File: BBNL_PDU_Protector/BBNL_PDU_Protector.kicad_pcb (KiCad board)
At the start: 2 copper layers, 107.3 x 39.4 mm, 20 parts, among them J1 1720796, J2 1708381

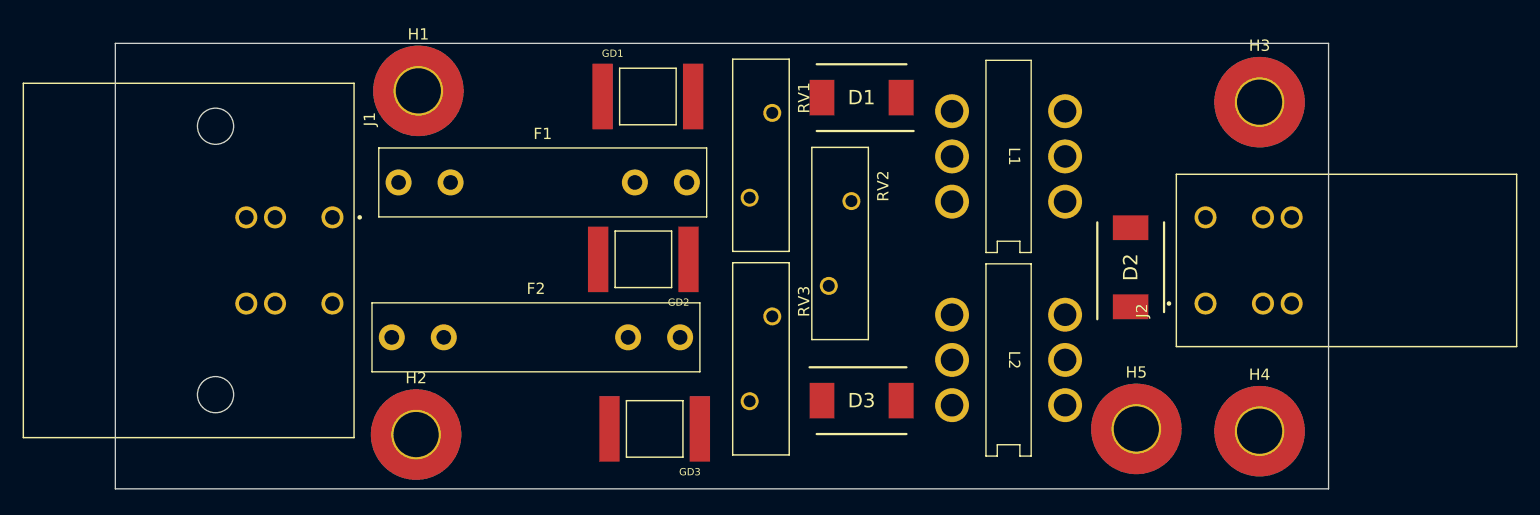
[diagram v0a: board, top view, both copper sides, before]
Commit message: second commit
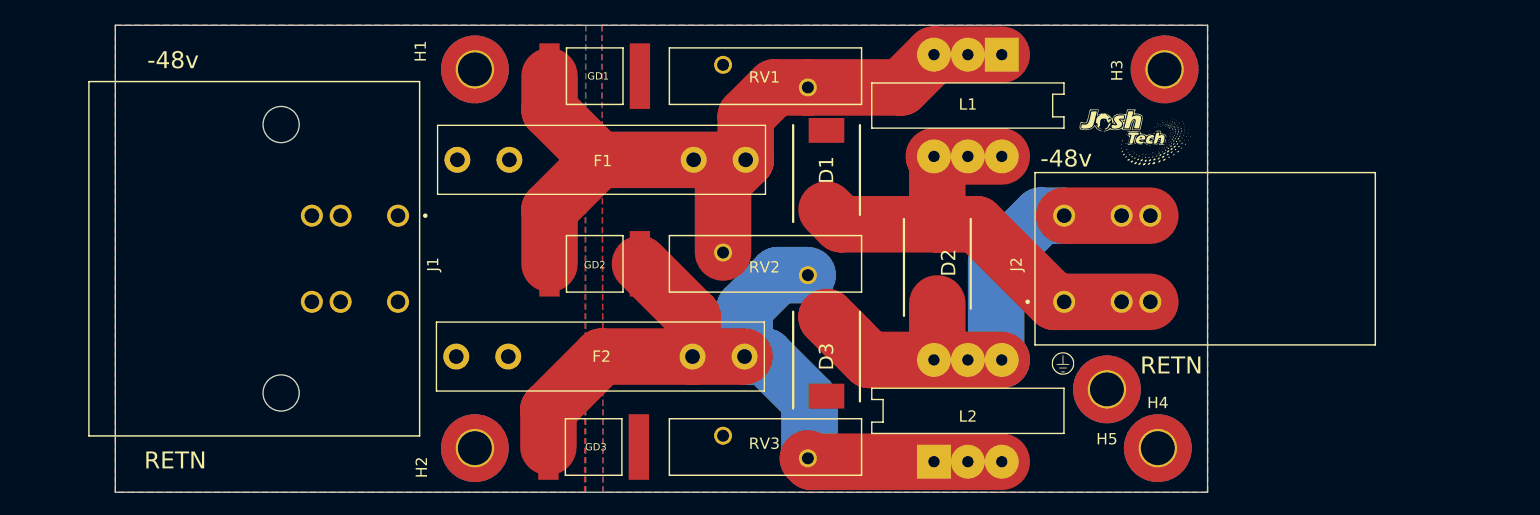
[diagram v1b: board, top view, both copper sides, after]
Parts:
- added G***: LOGO, PDU:GND, F.Cu at (140.8, 91.0)
- added G***: LOGO, PDU:JTS_logo, F.Cu at (147.2, 71.0)
- F1, F2: value Fuse -> 20A
- H1, H2, H3, H4, H5: footprint MountingHole:MountingHole_4mm_Pad_TopBottom -> MountingHole:MountingHole_3mm_Pad_TopBottom
- moved D2 17.1 mm to (129.7, 82.2)
- moved J2 12.5 mm to (168.4, 89.4)
- moved H4 9.12 mm to (149.2, 98.5)
- moved H3 8.89 mm to (149.8, 65.0)
- moved RV3 7.81 mm to (114.5, 98.4), turned to 180 degrees
- moved D1 7.11 mm to (119.9, 73.9), turned to 90 degrees
- moved RV1 7.01 mm to (114.5, 65.6), turned to 0 degrees
- moved RV2 6.84 mm to (114.5, 82.2), turned to 0 degrees
- moved F2 5.95 mm to (87.2, 90.4)
- moved J1 5.80 mm to (54.7, 66.1)
- moved L1 5.76 mm to (132.4, 68.2), turned to 0 degrees
- moved L2 5.76 mm to (132.4, 95.2), turned to 180 degrees
- moved GD3 5.63 mm to (99.3, 98.4)
- moved F1 5.57 mm to (87.2, 73.0)
- moved H1 5.35 mm to (88.8, 65.0)
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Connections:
- H1 pad 1: Earth -> unconnected-(H1-Pad1)
- H2 pad 1: Earth -> unconnected-(H2-Pad1)
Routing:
- net Net-(F2-Pad2): track 0.00 -> 73.6 mm
- net Net-(F1-Pad2): track 0.00 -> 71.0 mm
- net Net-(D2-Pad1): track 0.00 -> 49.5 mm
- net Net-(D1-Pad1): track 0.00 -> 44.1 mm
- added copper zone on B.Cu, net Earth
- added copper zone on F.Cu, net Earth
- added copper zone on F.Cu, net Net-(F1-Pad1)
- added copper zone on B.Cu, net Net-(F2-Pad1)
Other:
- board size 107.3 x 39.4 mm -> 96.6 x 41.3 mm
- board text added: "-48v"
- board text added: "RETN"
